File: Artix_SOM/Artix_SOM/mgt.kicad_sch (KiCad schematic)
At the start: 1 part, among them U1 XC7A100T-FGG676

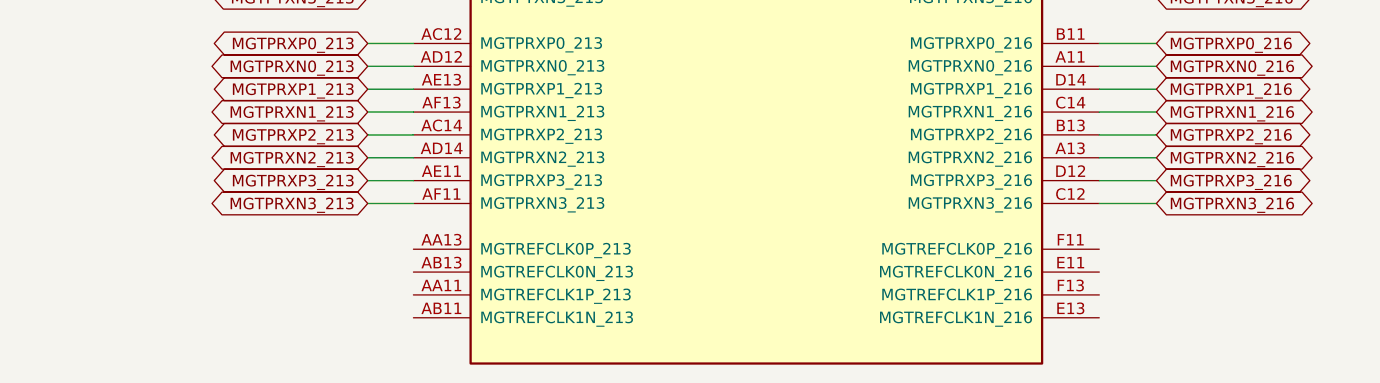
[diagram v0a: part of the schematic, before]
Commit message: update
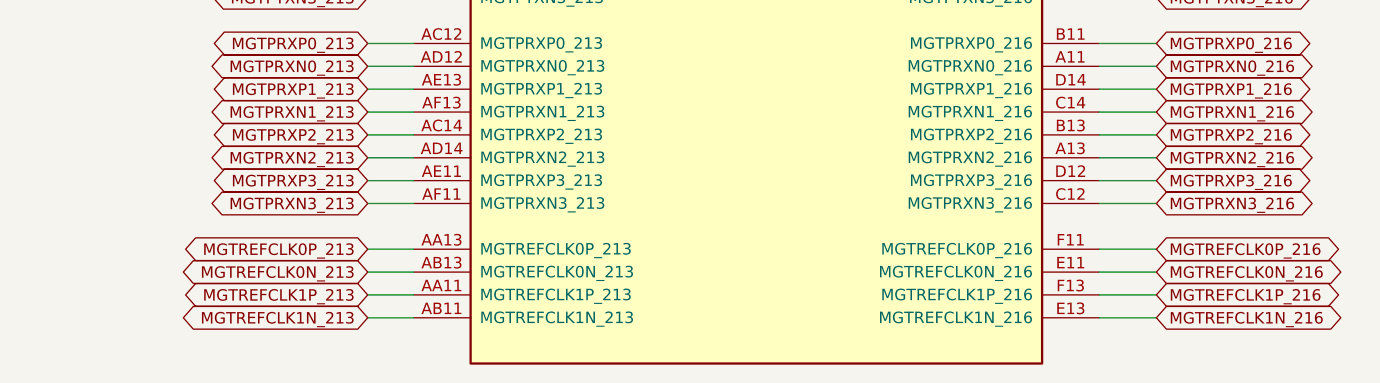
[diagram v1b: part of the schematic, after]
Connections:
- net MGTREFCLK1P_213: now reaches U1.AA11 (MGTREFCLK1P_213)
- net MGTREFCLK0P_213: now reaches U1.AA13 (MGTREFCLK0P_213)
- net MGTREFCLK1N_213: now reaches U1.AB11 (MGTREFCLK1N_213)
- net MGTREFCLK0N_213: now reaches U1.AB13 (MGTREFCLK0N_213)
- net MGTREFCLK0N_216: now reaches U1.E11 (MGTREFCLK0N_216)
- net MGTREFCLK1N_216: now reaches U1.E13 (MGTREFCLK1N_216)
- net MGTREFCLK0P_216: now reaches U1.F11 (MGTREFCLK0P_216)
- net MGTREFCLK1P_216: now reaches U1.F13 (MGTREFCLK1P_216)
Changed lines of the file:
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@@
+	(wire
+		(pts
+			(xy 328.93 147.32) (xy 322.58 147.32)
+		)
+		(stroke
+			(width 0)
+			(type default)
+		)
+	)
 	(wire
 		(pts
@@
 	(wire
 		(pts
+			(xy 241.3 152.4) (xy 246.38 152.4)
+		)
+		(stroke
+			(width 0)
+			(type default)
+		)
+	)
+	(wire
+		(pts
 			(xy 157.48 128.27) (xy 166.37 128.27)
 		)
@@
 	(wire
 		(pts
+			(xy 241.3 149.86) (xy 246.38 149.86)
+		)
+		(stroke
+			(width 0)
+			(type default)
+		)
+	)
+	(wire
+		(pts
 			(xy 72.39 113.03) (xy 72.39 115.57)
 		)
@@
 	(wire
 		(pts
+			(xy 328.93 152.4) (xy 322.58 152.4)
+		)
+		(stroke
+			(width 0)
+			(type default)
+		)
+	)
+	(wire
+		(pts
 			(xy 328.93 132.08) (xy 322.58 132.08)
 		)
@@
 	(wire
 		(pts
+			(xy 241.3 154.94) (xy 246.38 154.94)
+		)
+		(stroke
+			(width 0)
+			(type default)
+		)
+	)
+	(wire
+		(pts
 			(xy 241.3 137.16) (xy 246.38 137.16)
 		)
@@
 	(wire
 		(pts
+			(xy 241.3 147.32) (xy 246.38 147.32)
+		)
+		(stroke
+			(width 0)
+			(type default)
+		)
+	)
+	(wire
+		(pts
 			(xy 72.39 125.73) (xy 72.39 128.27)
 		)
@@
 	(wire
 		(pts
+			(xy 328.93 149.86) (xy 322.58 149.86)
+		)
+		(stroke
+			(width 0)
+			(type default)
+		)
+	)
+	(wire
+		(pts
 			(xy 157.48 123.19) (xy 166.37 123.19)
 		)
@@
 	(wire
 		(pts
+			(xy 328.93 154.94) (xy 322.58 154.94)
+		)
+		(stroke
+			(width 0)
+			(type default)
+		)
+	)
+	(wire
+		(pts
 			(xy 241.3 104.14) (xy 246.38 104.14)
 		)
@@
 		)
 	)
+	(global_label "MGTREFCLK1P_216"
+		(shape bidirectional)
+		(at 328.93 152.4 0)
+		(effects
+			(font
+				(size 1.27 1.27)
+			)
+			(justify left)
+		)
+		(property "Intersheetrefs" "${INTERSHEET_REFS}"
+			(at 328.93 152.4 0)
+			(effects
+				(font
+					(size 1.27 1.27)
+				)
+				(hide yes)
+			)
+		)
+	)
 	(global_label "MGTPRXN0_213"
 		(shape bidirectional)
@@
 		)
 	)
+	(global_label "MGTREFCLK0N_216"
+		(shape bidirectional)
+		(at 328.93 149.86 0)
+		(effects
+			(font
+				(size 1.27 1.27)
+			)
+			(justify left)
+		)
+		(property "Intersheetrefs" "${INTERSHEET_REFS}"
+			(at 328.93 149.86 0)
+			(effects
+				(font
+					(size 1.27 1.27)
+				)
+				(hide yes)
+			)
+		)
+	)
 	(global_label "MGTPRXP2_213"
 		(shape bidirectional)
@@
 		)
 	)
+	(global_label "MGTREFCLK0P_213"
+		(shape bidirectional)
+		(at 241.3 147.32 180)
+		(effects
+			(font
+				(size 1.27 1.27)
+			)
+			(justify right)
+		)
+		(property "Intersheetrefs" "${INTERSHEET_REFS}"
+			(at 241.3 147.32 0)
+			(effects
+				(font
+					(size 1.27 1.27)
+				)
+				(hide yes)
+			)
+		)
+	)
+	(global_label "MGTREFCLK1N_213"
+		(shape bidirectional)
+		(at 241.3 154.94 180)
+		(effects
+			(font
+				(size 1.27 1.27)
+			)
+			(justify right)
+		)
+		(property "Intersheetrefs" "${INTERSHEET_REFS}"
+			(at 241.3 154.94 0)
+			(effects
+				(font
+					(size 1.27 1.27)
+				)
+				(hide yes)
+			)
+		)
+	)
 	(global_label "MGTPRXN1_213"
 		(shape bidirectional)
@@
 		)
 	)
+	(global_label "MGTREFCLK0P_216"
+		(shape bidirectional)
+		(at 328.93 147.32 0)
+		(effects
+			(font
+				(size 1.27 1.27)
+			)
+			(justify left)
+		)
+		(property "Intersheetrefs" "${INTERSHEET_REFS}"
+			(at 328.93 147.32 0)
+			(effects
+				(font
+					(size 1.27 1.27)
+				)
+				(hide yes)
+			)
+		)
+	)
 	(global_label "MGTPRXP1_213"
 		(shape bidirectional)
@@
 		)
 	)
+	(global_label "MGTREFCLK0N_213"
+		(shape bidirectional)
+		(at 241.3 149.86 180)
+		(effects
+			(font
+				(size 1.27 1.27)
+			)
+			(justify right)
+		)
+		(property "Intersheetrefs" "${INTERSHEET_REFS}"
+			(at 241.3 149.86 0)
+			(effects
+				(font
+					(size 1.27 1.27)
+				)
+				(hide yes)
+			)
+		)
+	)
 	(global_label "MGTPTXP3_213"
 		(shape bidirectional)
@@
 		)
 	)
+	(global_label "MGTREFCLK1P_213"
+		(shape bidirectional)
+		(at 241.3 152.4 180)
+		(effects
+			(font
+				(size 1.27 1.27)
+			)
+			(justify right)
+		)
+		(property "Intersheetrefs" "${INTERSHEET_REFS}"
+			(at 241.3 152.4 0)
+			(effects
+				(font
+					(size 1.27 1.27)
+				)
+				(hide yes)
+			)
+		)
+	)
 	(global_label "MGTPTXN0_216"
 		(shape bidirectional)
@@
 			(effects
 				(font
+					(size 1.27 1.27)
+				)
+				(hide yes)
+			)
+		)
+	)
+	(global_label "MGTREFCLK1N_216"
+		(shape bidirectional)
+		(at 328.93 154.94 0)
+		(effects
+			(font
+				(size 1.27 1.27)
+			)
+			(justify left)
+		)
+		(property "Intersheetrefs" "${INTERSHEET_REFS}"
+			(at 328.93 154.94 0)
+			(effects
+				(font
